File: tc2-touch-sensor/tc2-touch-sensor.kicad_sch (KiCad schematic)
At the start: 23 parts, among them J301 Screw_Terminal_01x01, J302 Conn_02x03_Odd_Even, J303 Screw_Terminal_01x01, Q301 AO3400A, U301 ME6216A28XG, U302 AT42QT1010-TSHR

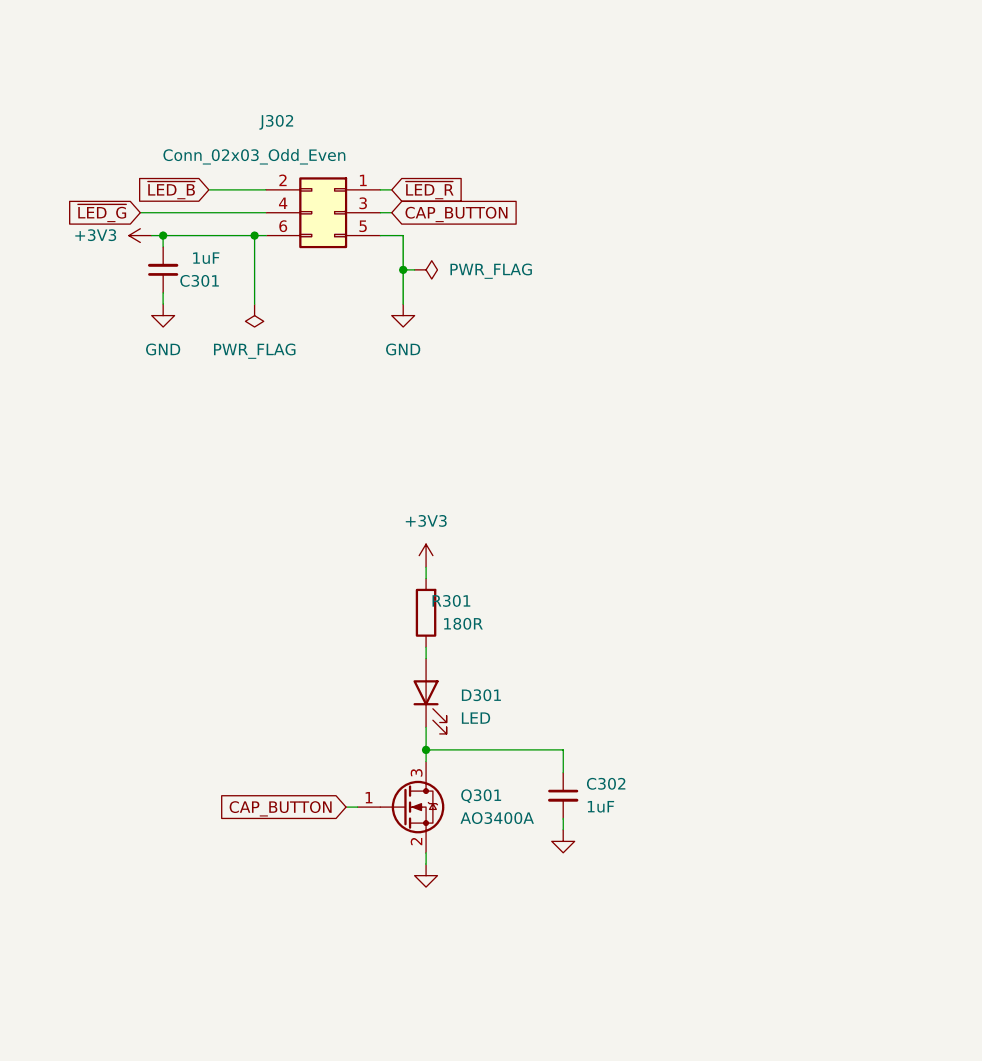
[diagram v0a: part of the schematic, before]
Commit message: Small updates
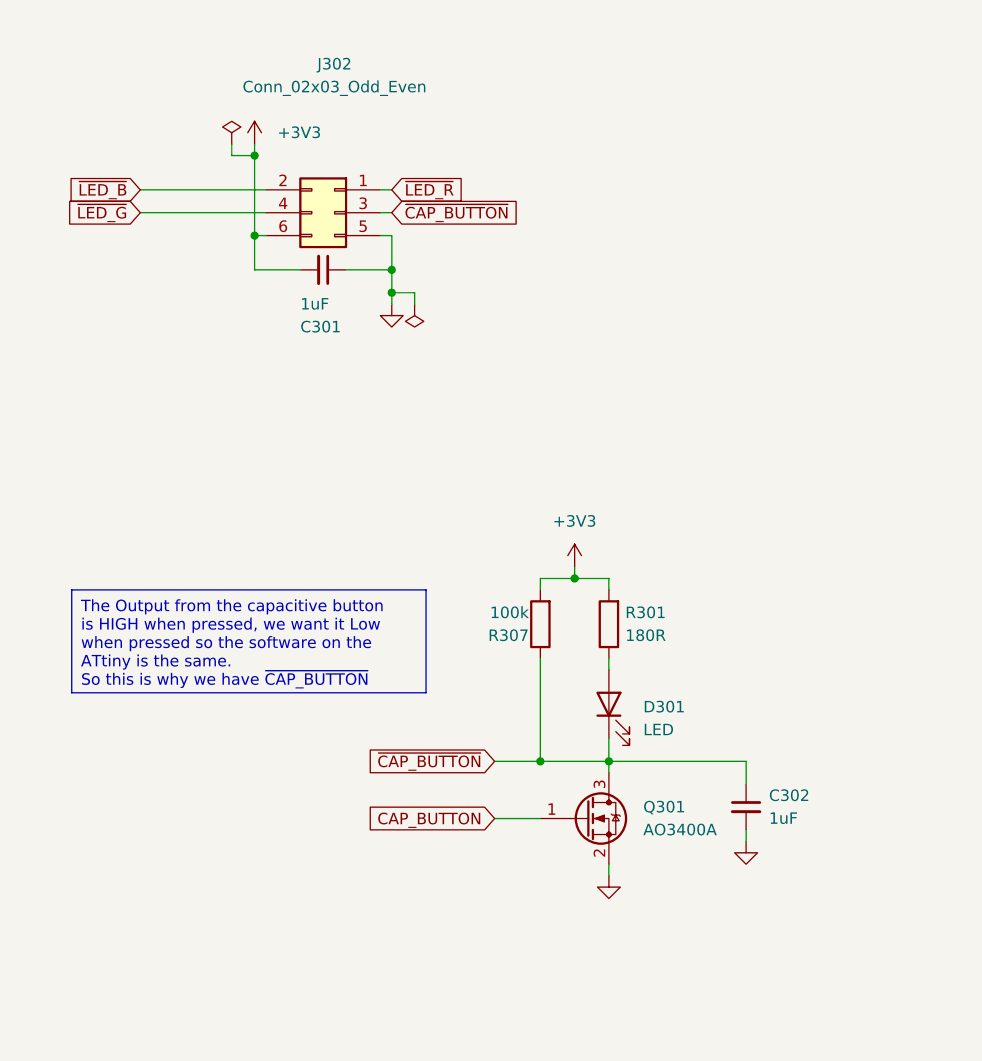
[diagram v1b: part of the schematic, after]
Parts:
- added R307: 100k, Resistor_SMD:R_0402_1005Metric, symbol Device:R
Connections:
- net +3V3: now also R307.2
- net CAP_BUTTON: no longer J302.3 (Pin_3)
- net ~{CAP_BUTTON}: now reaches C302.1, D301.1 (K), Q301.3 (D)
- net ~{CAP_BUTTON}: now also J302.3 (Pin_3), R307.1
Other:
- moved on the sheet: C301, C302, D301, Q301, R301
